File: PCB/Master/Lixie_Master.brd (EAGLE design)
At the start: 52 x 50 mm, 19 parts, among them IC1 FT232RL, J1 65100516121

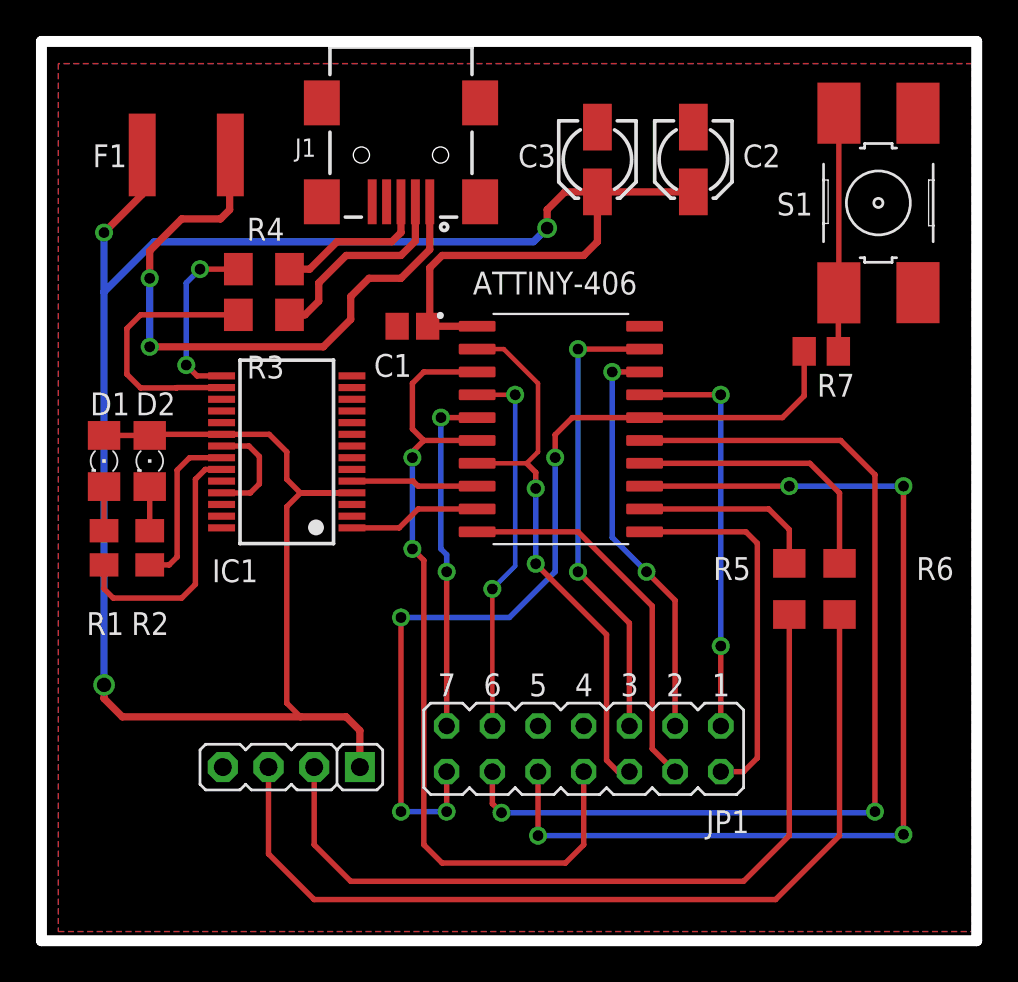
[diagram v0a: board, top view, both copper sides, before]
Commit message: V06
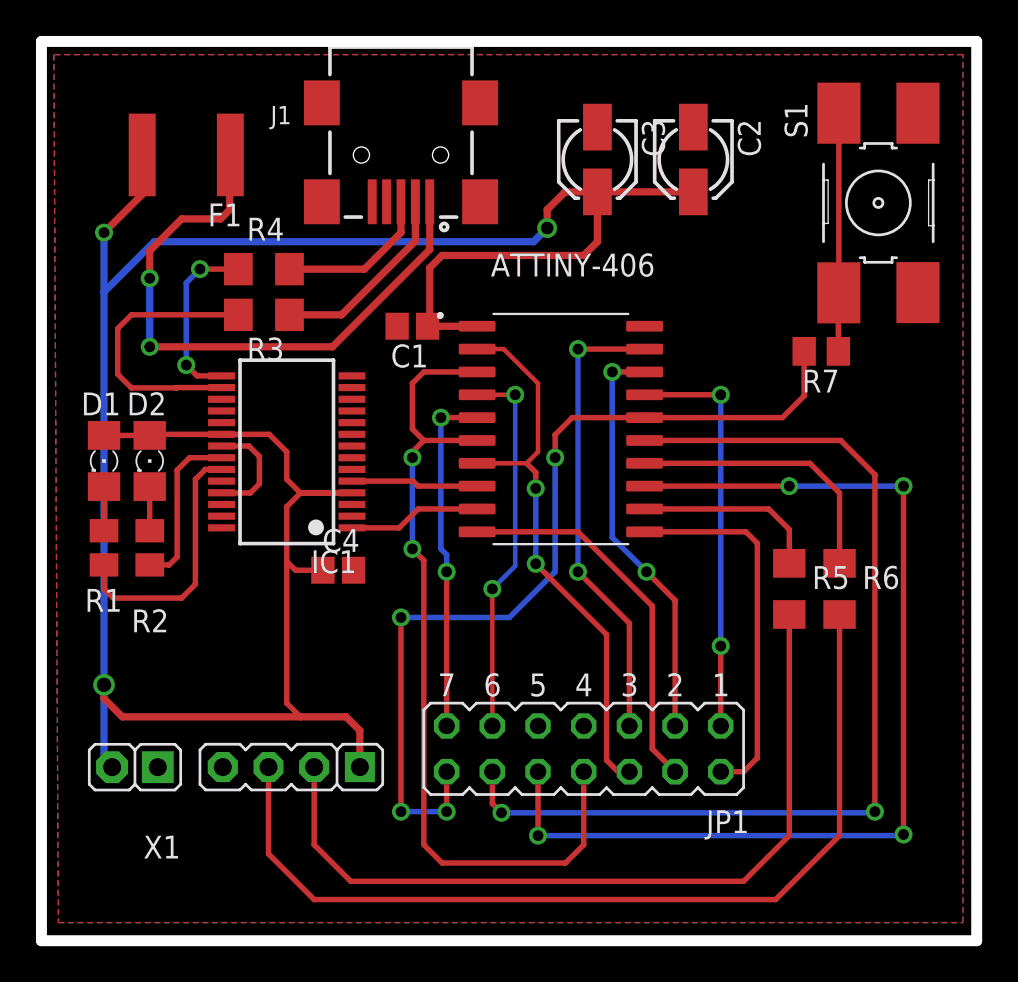
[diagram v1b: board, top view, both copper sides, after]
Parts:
- added C4: 0u1, 0_HTL_MegaCard_V3:C0805
- added X1: PIN2", 0_HTL_uC-MEGACARD:PIN2
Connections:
- net GND: now also C4.2, X1.P$2
- net VCC: now also C4.1, X1.P$3
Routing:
- net VCC: track 134.8 -> 141.8 mm
- net N$2: track 14.6 -> 15.7 mm
- net N$14: track 35.0 -> 34.3 mm
- net N$4: track 11.5 -> 10.9 mm
